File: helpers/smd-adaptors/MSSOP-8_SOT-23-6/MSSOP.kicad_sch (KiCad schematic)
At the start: 4 parts, among them J1 Conn_01x05, J2 Conn_01x05, J3 Conn_01x10, J4 Conn_01x10

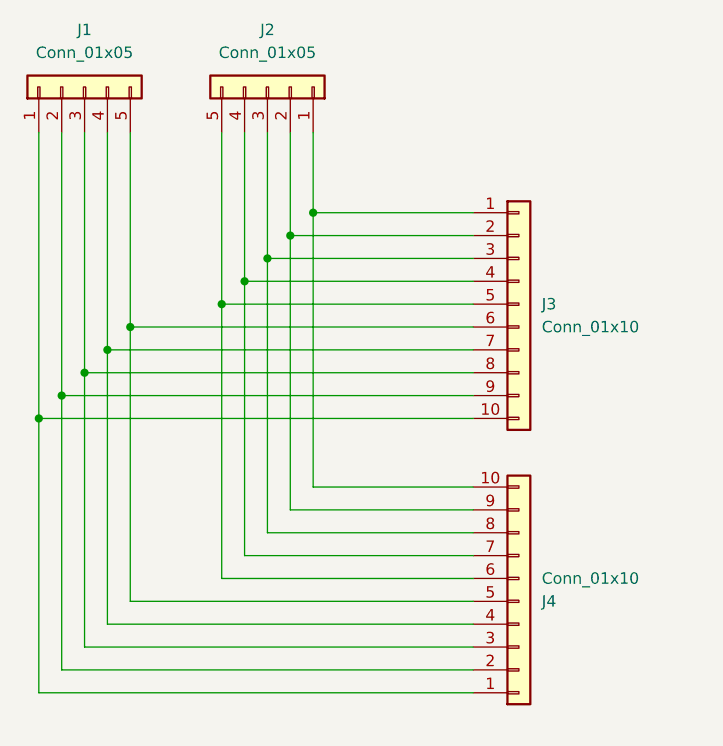
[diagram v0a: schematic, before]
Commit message: firmware for midas, quantizer updates
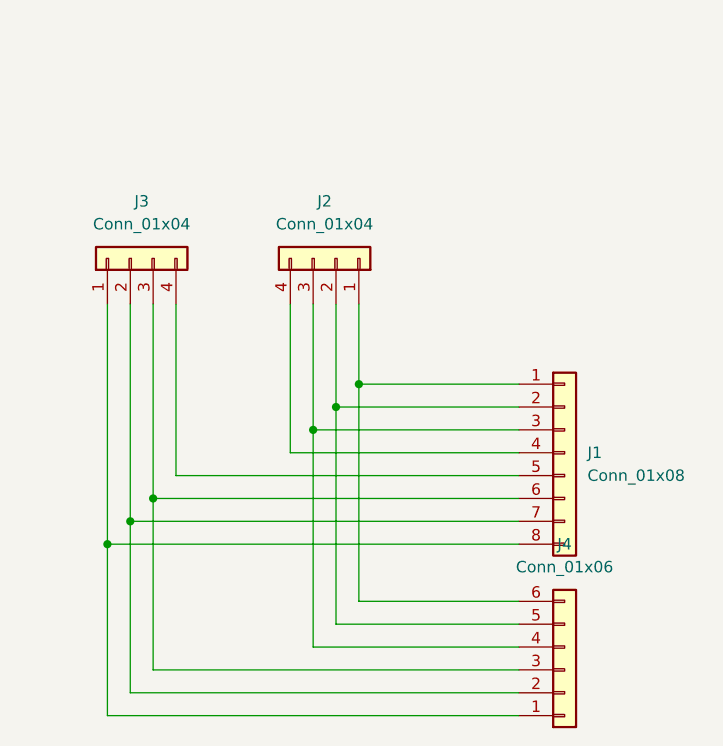
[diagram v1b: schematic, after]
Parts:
- removed J1, J2: Conn_01x05, Connector_PinHeader_2.54mm:PinHeader_1x05_P2.54mm_Vertical, symbol Connector_Generic:Conn_01x05
- removed J3: Conn_01x10, Package_SO:MSOP-10_3x3mm_P0.5mm, symbol Connector_Generic:Conn_01x10
- removed J4: Conn_01x10, Package_SO:SOIC-10_3.9x4.9mm_P1mm, symbol Connector_Generic:Conn_01x10
- added J1: Conn_01x08, Package_SO:MSOP-8_3x3mm_P0.65mm, symbol Connector_Generic:Conn_01x08
- added J2, J3: Conn_01x04, Synth:PinHeader_1x04_P2.54mm_Vertical, symbol Connector_Generic:Conn_01x04
- added J4: Conn_01x06, Package_TO_SOT_SMD:SOT-23-6_Handsoldering, symbol Connector_Generic:Conn_01x06
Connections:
- new net: J1.1 (Pin_1), J2.1 (Pin_1), J4.6 (Pin_6)
- new net: J1.2 (Pin_2), J2.2 (Pin_2), J4.5 (Pin_5)
- new net: J1.3 (Pin_3), J2.3 (Pin_3), J4.4 (Pin_4)
- new net: J1.4 (Pin_4), J2.4 (Pin_4)
- new net: J1.5 (Pin_5), J3.4 (Pin_4)
- new net: J1.6 (Pin_6), J3.3 (Pin_3), J4.3 (Pin_3)
- new net: J1.7 (Pin_7), J3.2 (Pin_2), J4.2 (Pin_2)
- new net: J1.8 (Pin_8), J3.1 (Pin_1), J4.1 (Pin_1)
